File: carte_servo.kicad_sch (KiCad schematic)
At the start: 39 parts, among them J16 Conn_01x04_Male, J17 Conn_01x04_Male, J2 Conn_02x04_Top_Bottom, J24 Conn_LEDs, P1 USB_C_Plug_USB2.0, SW1 CK_KMS2xxG, U1 XGZP6897D_differential_pressu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, U2 XGZP6897D_differential_pressu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, U6 SN65HVD230, U7 LD1117S33TR_SOT223, U8 ESP32-S3-WROOM-1

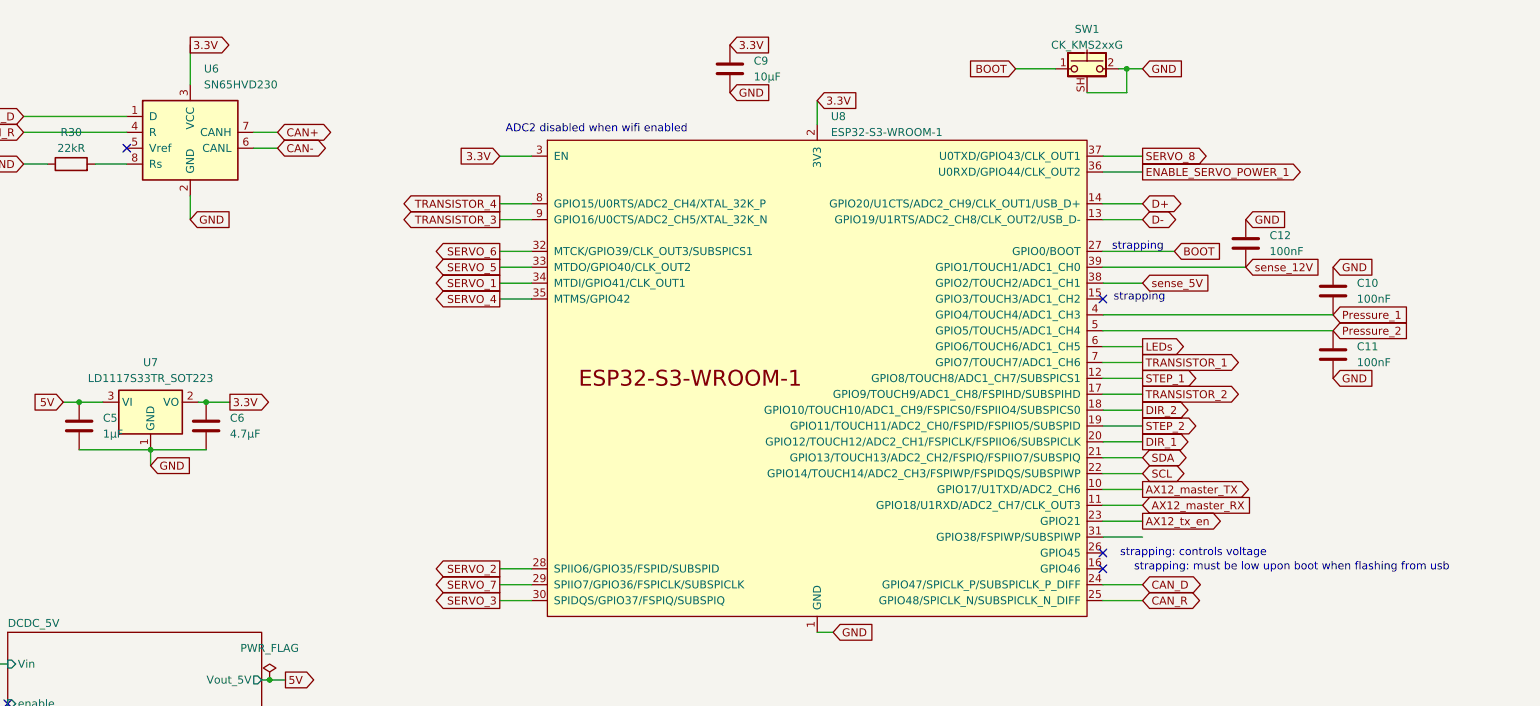
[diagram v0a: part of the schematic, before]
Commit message: continue routing
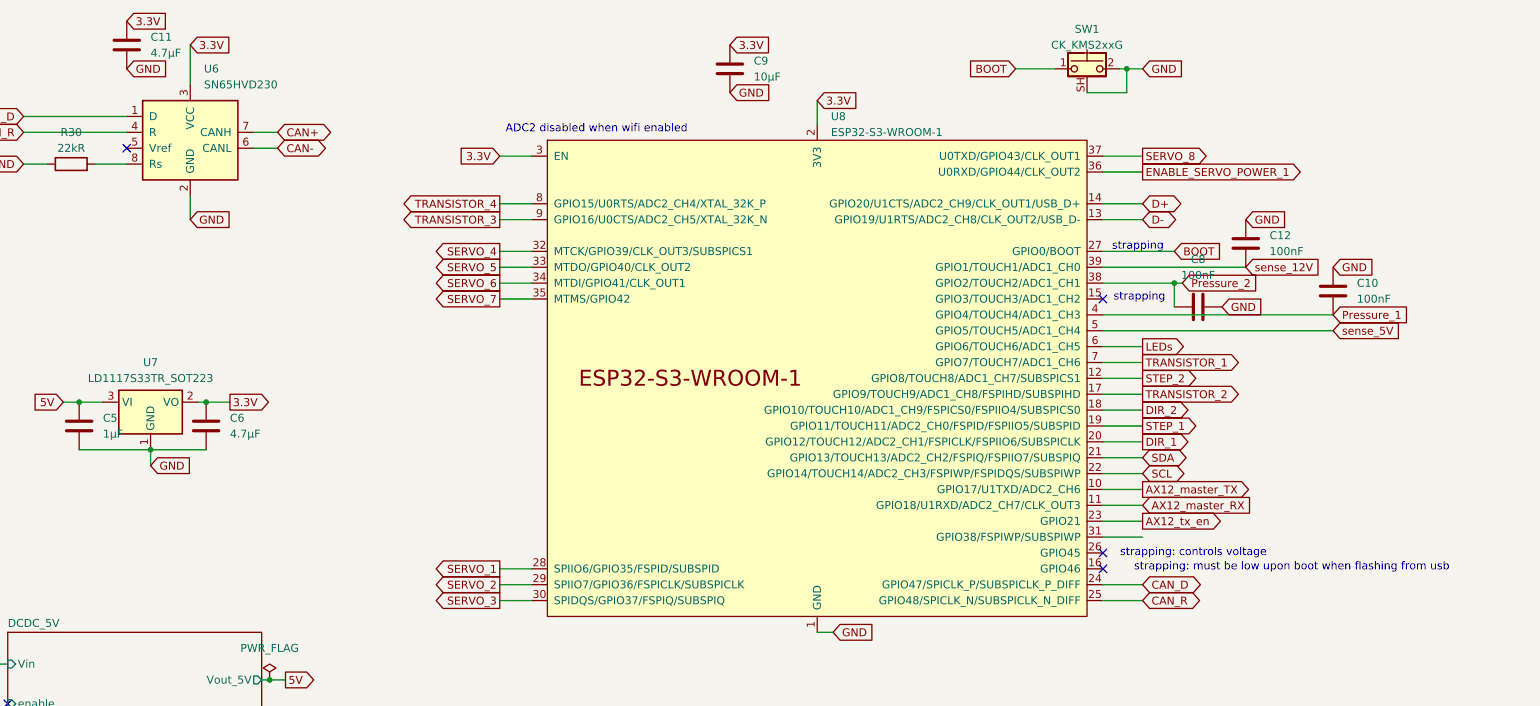
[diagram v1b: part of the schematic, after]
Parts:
- added C8: 100nF, Capacitor_SMD:C_0603_1608Metric, symbol Device:C
- C11: value 100nF -> 4.7µF
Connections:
- net 3.3V: now also C11.1
- net GND: now also C8.2
- net Pressure_2: now also U8.38 (GPIO2/TOUCH2/ADC1_CH1), C8.1; no longer C11.1, U8.5 (GPIO5/TOUCH5/ADC1_CH4)
- net SERVO_1: now also U8.28 (SPIIO6/GPIO35/FSPID/SUBSPID); no longer U8.34 (MTDI/GPIO41/CLK_OUT1)
- net SERVO_2: now also U8.29 (SPIIO7/GPIO36/FSPICLK/SUBSPICLK); no longer U8.28 (SPIIO6/GPIO35/FSPID/SUBSPID)
- net SERVO_4: now also U8.32 (MTCK/GPIO39/CLK_OUT3/SUBSPICS1); no longer U8.35 (MTMS/GPIO42)
- net SERVO_6: now also U8.34 (MTDI/GPIO41/CLK_OUT1); no longer U8.32 (MTCK/GPIO39/CLK_OUT3/SUBSPICS1)
- net SERVO_7: now also U8.35 (MTMS/GPIO42); no longer U8.29 (SPIIO7/GPIO36/FSPICLK/SUBSPICLK)
- net STEP_1: now also U8.19 (GPIO11/TOUCH11/ADC2_CH0/FSPID/FSPIIO5/SUBSPID); no longer U8.12 (GPIO8/TOUCH8/ADC1_CH7/SUBSPICS1)
- net STEP_2: now also U8.12 (GPIO8/TOUCH8/ADC1_CH7/SUBSPICS1); no longer U8.19 (GPIO11/TOUCH11/ADC2_CH0/FSPID/FSPIIO5/SUBSPID)
- net sense_5V: now also U8.5 (GPIO5/TOUCH5/ADC1_CH4); no longer U8.38 (GPIO2/TOUCH2/ADC1_CH1)

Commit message: basic routing
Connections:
- net DIR_2: now also U8.6 (GPIO6/TOUCH6/ADC1_CH5); no longer U8.18 (GPIO10/TOUCH10/ADC1_CH9/FSPICS0/FSPIIO4/SUBSPICS0)
- net LEDs: now also U8.18 (GPIO10/TOUCH10/ADC1_CH9/FSPICS0/FSPIIO4/SUBSPICS0); no longer U8.6 (GPIO6/TOUCH6/ADC1_CH5)
- net SCL: no longer U2.7 (SCL)
- net SDA: no longer U2.6 (SDA)
- no-connect marks 8 -> 10
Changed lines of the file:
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@@
 	)
 	(no_connect
+		(at 107.95 127)
+	)
+	(no_connect
 		(at 331.47 12.7)
 	)
@@
 	)
 	(no_connect
+		(at 107.95 124.46)
+	)
+	(no_connect
 		(at 487.68 80.01)
 	)
@@
 	(wire
 		(pts
-			(xy 107.95 127) (xy 115.57 127)
-		)
-		(stroke
-			(width 0)
-			(type default)
-		)
-	)
-	(wire
-		(pts
 			(xy 355.6 10.16) (xy 351.79 10.16)
 		)
@@
 	(wire
 		(pts
-			(xy 107.95 124.46) (xy 115.57 124.46)
-		)
-		(stroke
-			(width 0)
-			(type default)
-		)
-	)
-	(wire
-		(pts
 			(xy 125.73 177.8) (xy 127 177.8)
 		)
@@
 	(label "Pressure_2"
 		(at 83.82 127 180)
+		(fields_autoplaced yes)
 		(effects
 			(font
@@
 	(label "Pressure_1"
 		(at 82.55 100.33 180)
+		(fields_autoplaced yes)
 		(effects
 			(font
@@
 		)
 	)
+	(global_label "LEDs"
+		(shape output)
+		(at 494.03 54.61 0)
+		(fields_autoplaced yes)
+		(effects
+			(font
+				(size 1.27 1.27)
+			)
+			(justify left)
+		)
+		(property "Intersheetrefs" "${INTERSHEET_REFS}"
+			(at 501.4904 54.61 0)
+			(effects
+				(font
+					(size 1.27 1.27)
+				)
+				(justify left)
+				(hide yes)
+			)
+		)
+	)
 	(global_label "5V"
 		(shape input)
@@
 		)
 	)
-	(global_label "SDA"
-		(shape input)
-		(at 115.57 127 0)
-		(fields_autoplaced yes)
-		(effects
-			(font
-				(size 1.27 1.27)
-			)
-			(justify left)
-		)
-		(property "Intersheetrefs" "${INTERSHEET_REFS}"
-			(at 121.5512 126.9206 0)
-			(effects
-				(font
-					(size 1.27 1.27)
-				)
-				(justify left)
-				(hide yes)
-			)
-		)
-	)
 	(global_label "SERVO_6"
 		(shape output)
@@
 		)
 	)
-	(global_label "DIR_2"
-		(shape output)
-		(at 494.03 54.61 0)
-		(fields_autoplaced yes)
-		(effects
-			(font
-				(size 1.27 1.27)
-			)
-			(justify left)
-		)
-		(property "Intersheetrefs" "${INTERSHEET_REFS}"
-			(at 502.3371 54.61 0)
-			(effects
-				(font
-					(size 1.27 1.27)
-				)
-				(justify left)
-				(hide yes)
-			)
-		)
-	)
 	(global_label "GND"
 		(shape input)
@@
 		)
 	)
+	(global_label "DIR_2"
+		(shape output)
+		(at 494.03 44.45 0)
+		(fields_autoplaced yes)
+		(effects
+			(font
+				(size 1.27 1.27)
+			)
+			(justify left)
+		)
+		(property "Intersheetrefs" "${INTERSHEET_REFS}"
+			(at 502.3371 44.45 0)
+			(effects
+				(font
+					(size 1.27 1.27)
+				)
+				(justify left)
+				(hide yes)
+			)
+		)
+	)
 	(global_label "12V_POW_P"
 		(shape input)
@@
 		)
 	)
-	(global_label "CAN+"
-		(shape bidirectional)
-		(at 355.6 10.16 0)
+	(global_label "STEP_2"
+		(shape output)
+		(at 494.03 49.53 0)
 		(fields_autoplaced yes)
 		(effects
@@
 		)
 		(property "Intersheetrefs" "${INTERSHEET_REFS}"
-			(at 364.958 10.16 0)
+			(at 503.7884 49.53 0)
 			(effects
 				(font
@@
 		)
 	)
-	(global_label "LEDs"
-		(shape output)
-		(at 494.03 44.45 0)
+	(global_label "CAN+"
+		(shape bidirectional)
+		(at 355.6 10.16 0)
 		(fields_autoplaced yes)
 		(effects
@@
 		)
 		(property "Intersheetrefs" "${INTERSHEET_REFS}"
-			(at 501.4904 44.45 0)
+			(at 364.958 10.16 0)
 			(effects
 				(font
@@
 		)
 	)
-	(global_label "SCL"
-		(shape input)
-		(at 115.57 124.46 0)
-		(fields_autoplaced yes)
-		(effects
-			(font
-				(size 1.27 1.27)
-			)
-			(justify left)
-		)
-		(property "Intersheetrefs" "${INTERSHEET_REFS}"
-			(at 121.4907 124.3806 0)
-			(effects
-				(font
-					(size 1.27 1.27)
-				)
-				(justify left)
-				(hide yes)
-			)
-		)
-	)
 	(global_label "SERVO_5"
 		(shape output)
@@
 				(hide yes)
 			)
-		)
-	)
-	(global_label "STEP_2"
-		(shape output)
-		(at 494.03 49.53 0)
-		(fields_autoplaced yes)
-		(effects
-			(font
-				(size 1.27 1.27)
-			)
-			(justify left)
-		)
-		(property "Intersheetrefs" "${INTERSHEET_REFS}"
-			(at 503.7884 49.53 0)
-			(effects
-				(font
-					(size 1.27 1.27)
-				)
-				(justify left)
-				(hide yes)
-			)
